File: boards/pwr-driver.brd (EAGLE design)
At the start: 99 x 56 mm, 27 parts

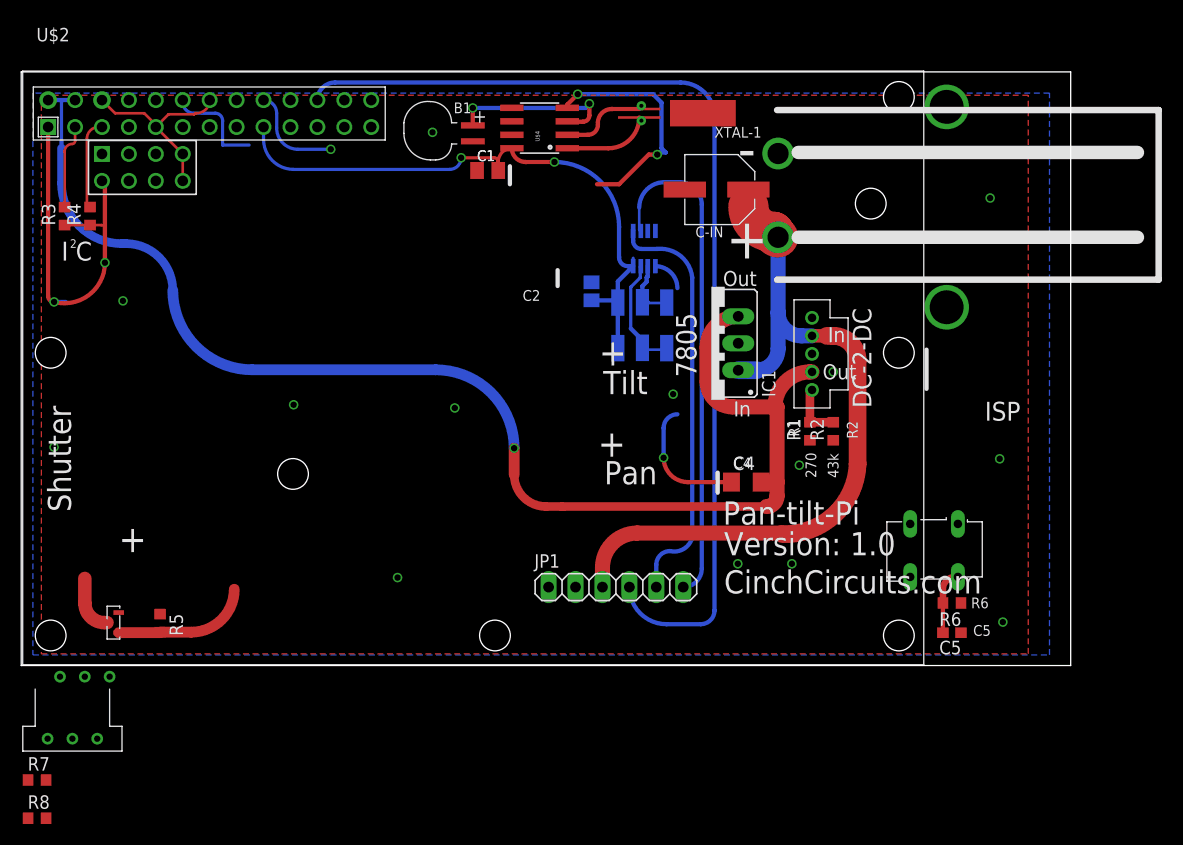
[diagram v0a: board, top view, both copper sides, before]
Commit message: Added more parts and a readme.
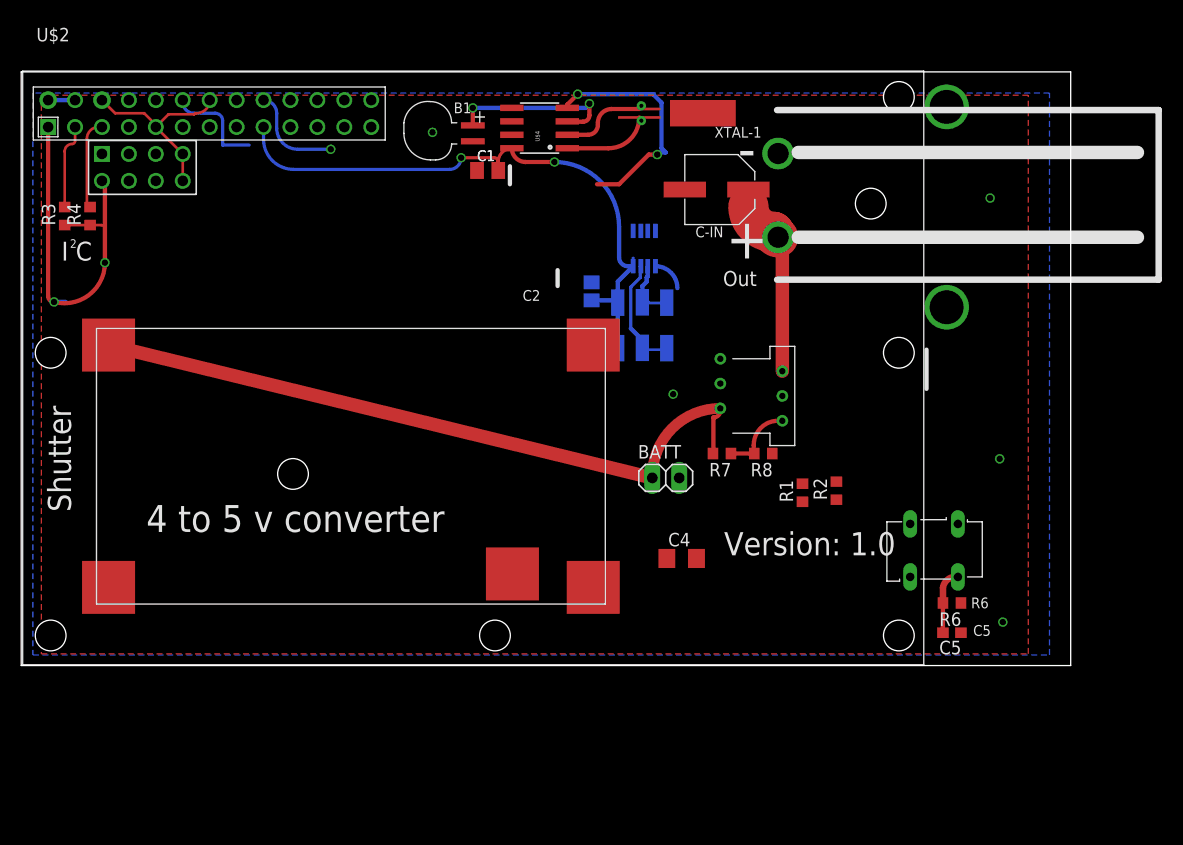
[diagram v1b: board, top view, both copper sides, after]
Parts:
- removed IC1: (no value), v-reg:78XXS
- removed JP1: (no value), pinhead:1X06
- removed R5: 10k, resistor:R0603
- removed U$10: NPN-T-SMALL, mgregg:SOT23
- removed U$7: OKR-T-W12-DC-TO-DC, mgregg:OKR-T-W12
- added BATT: (no value), pinhead:1X02
- added U$3: STEP-UP-FROM-AMAZON, needed-parts:STEP-UP-FROM-AMAZON
- moved R8 76.7 mm to (70.0, 20.0), turned to 180 degrees
- moved U$1 73.8 mm to (71.8, 26.6), turned to 90 degrees
- moved R7 71.6 mm to (66.1, 20.0), turned to 180 degrees
- moved C4 9.44 mm to (62.3, 10.1)
- moved R1 5.84 mm to (73.7, 16.3)
- moved R2 5.61 mm to (76.9, 16.5)
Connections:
- removed net N$15: U$1.P$6
- removed net N$8: U$7.REMOTE
- removed net SCREEN1: U$10.P$3
- net 3V3: no longer JP1.2
- net 5V: now also U$3.OUT+; no longer IC1.OUT, U$7.VOUT
- net BATT: now also BATT.1, U$1.P$6, U$3.IN+
- net GND: now also BATT.2, U$3.GND, U$3.IN-, U$3.OUT-; no longer IC1.GND, JP1.1, R5.1, U$10.P$2, U$7.GND
- net GPIO25: no longer JP1.4
- net SCL: no longer JP1.6
- net SCREEN: no longer R5.2, U$10.P$1
- net SDA: no longer JP1.5
- net TRIM: no longer U$7.TRIM
- net VIN: no longer IC1.IN, JP1.3, U$7.VIN
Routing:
- net 5V: track 123.8 -> 2.54 mm, vias 1 -> 0
- net GPIO25: track 96.1 -> 0.00 mm
- net BATT: track 0.00 -> 66.6 mm
- net VIN: track 75.9 -> 18.5 mm
- net SCL: track 55.6 -> 8.70 mm
- net SDA: track 46.8 -> 8.13 mm
- net SCREEN: track 12.6 -> 0.00 mm
- net GND: track 56.0 -> 44.0 mm, vias 17 -> 7
- net N$4: track 0.00 -> 6.67 mm
- net TRIM: track 5.33 -> 0.00 mm
- net SCREEN1: track 5.19 -> 0.00 mm
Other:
- board text added: "4 to 5 v converter"
- board text removed: "270"
- board text removed: "43k"
- board text removed: "7805"
- board text removed: "C4"
- board text removed: "CinchCircuits.com"
- board text removed: "DC-2-DC"
- board text removed: "ISP"
- board text removed: "In"
- board text removed: "Max Input Voltage Dependant on C-IN."
- board text removed: "Pan"
- board text removed: "Pan-tilt-Pi"
- board text removed: "R1"
- board text removed: "R2"
- board text removed: "Tilt"
